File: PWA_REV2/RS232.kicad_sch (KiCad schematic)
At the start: 19 parts

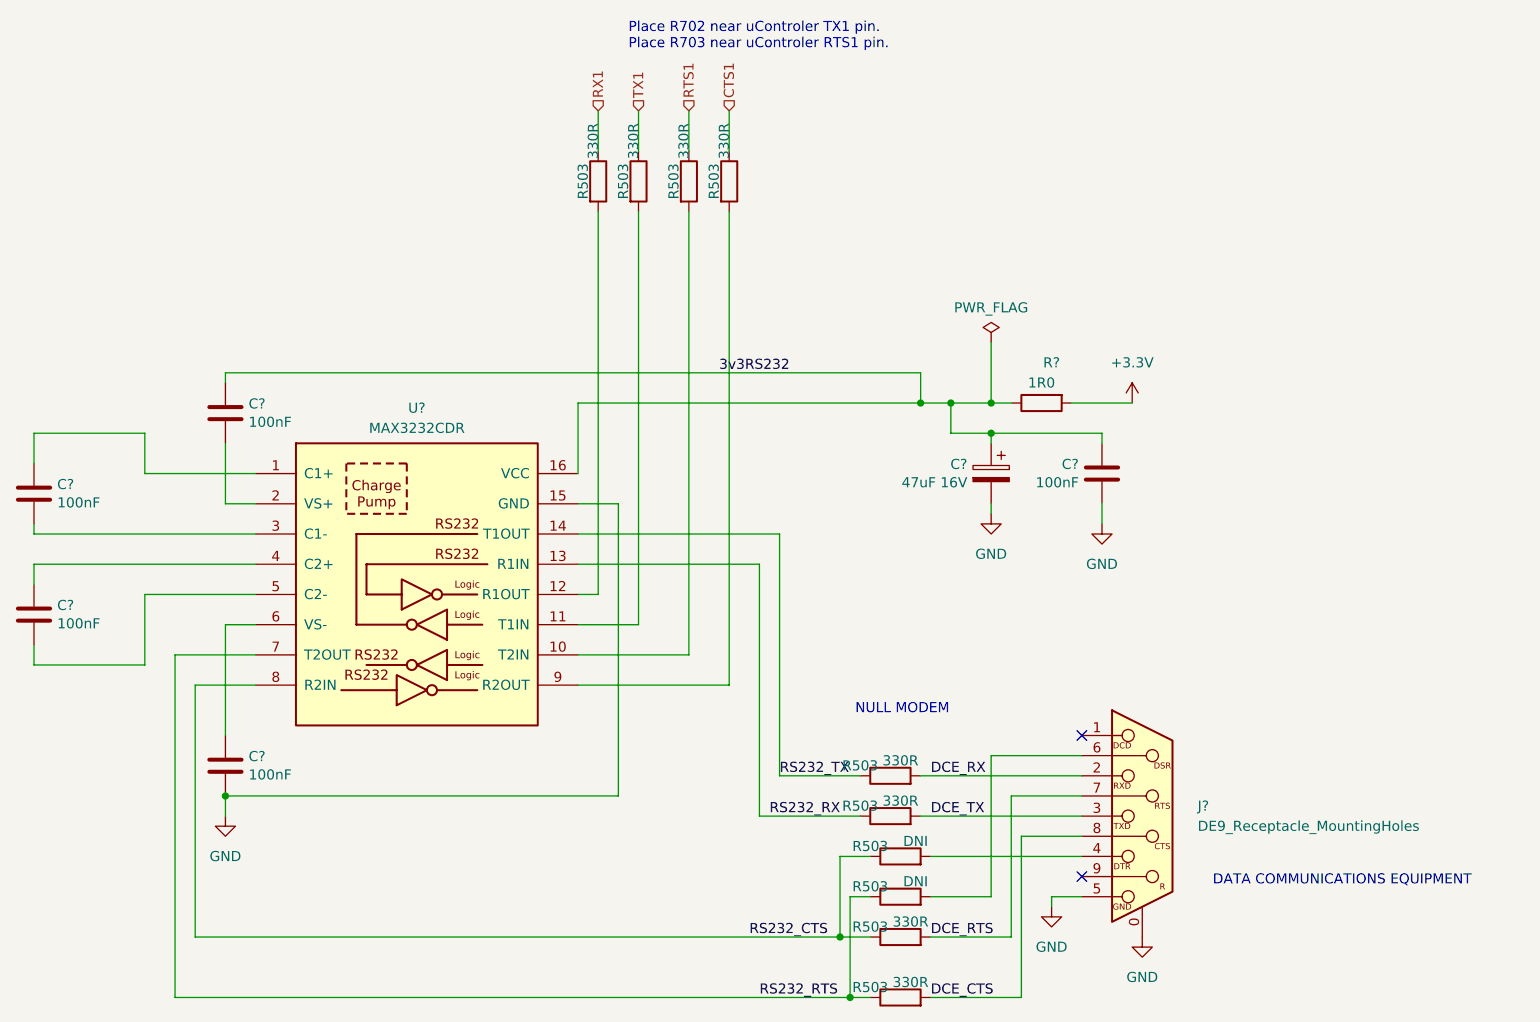
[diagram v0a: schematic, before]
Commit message: Hardware, PWA, Add a Jumper to BOM for J102 so that USB Connector Can Power Krake, issue 312.
:q
q
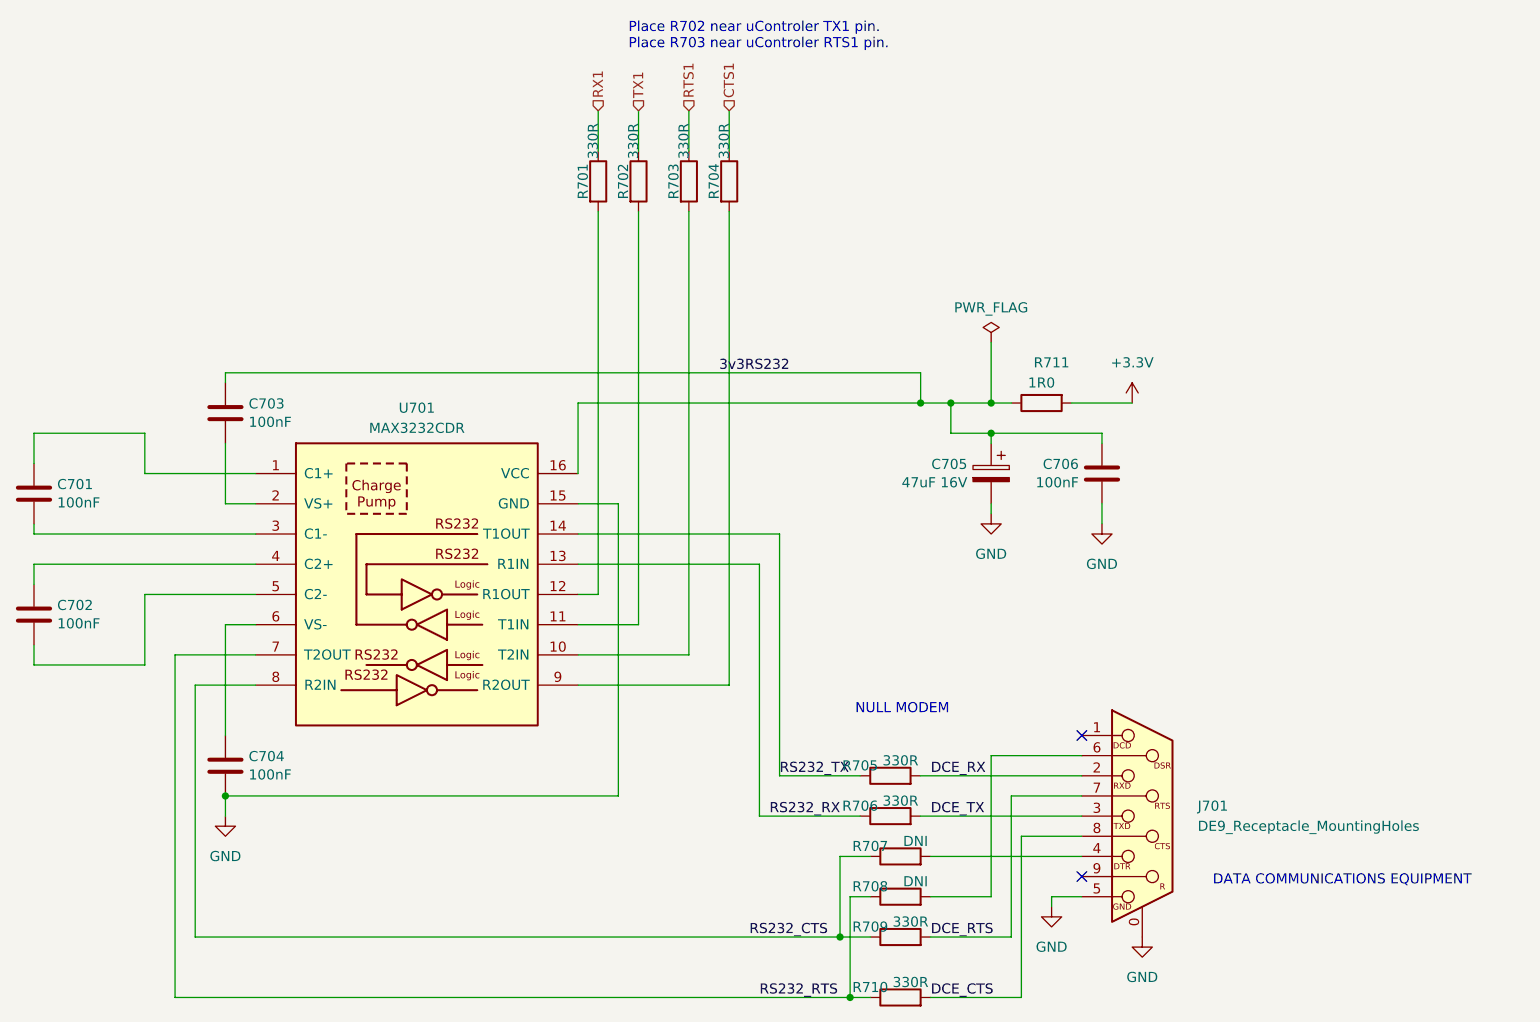
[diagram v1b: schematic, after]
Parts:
- gave numbers to parts that had none: 9
- renumbered R503 to R701, R503 to R702, R503 to R703, R503 to R704, R503 to R705, R503 to R706, R503 to R707, R503 to R708, R503 to R709, R503 to R710

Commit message: Revert "Hardware, PWA, Add a Jumper to BOM for J102 so that USB Connector Can Power Krake, issue 312."
This reverts commit c2819b8ee4999f733f52d823f88f6aefd6456fcc.
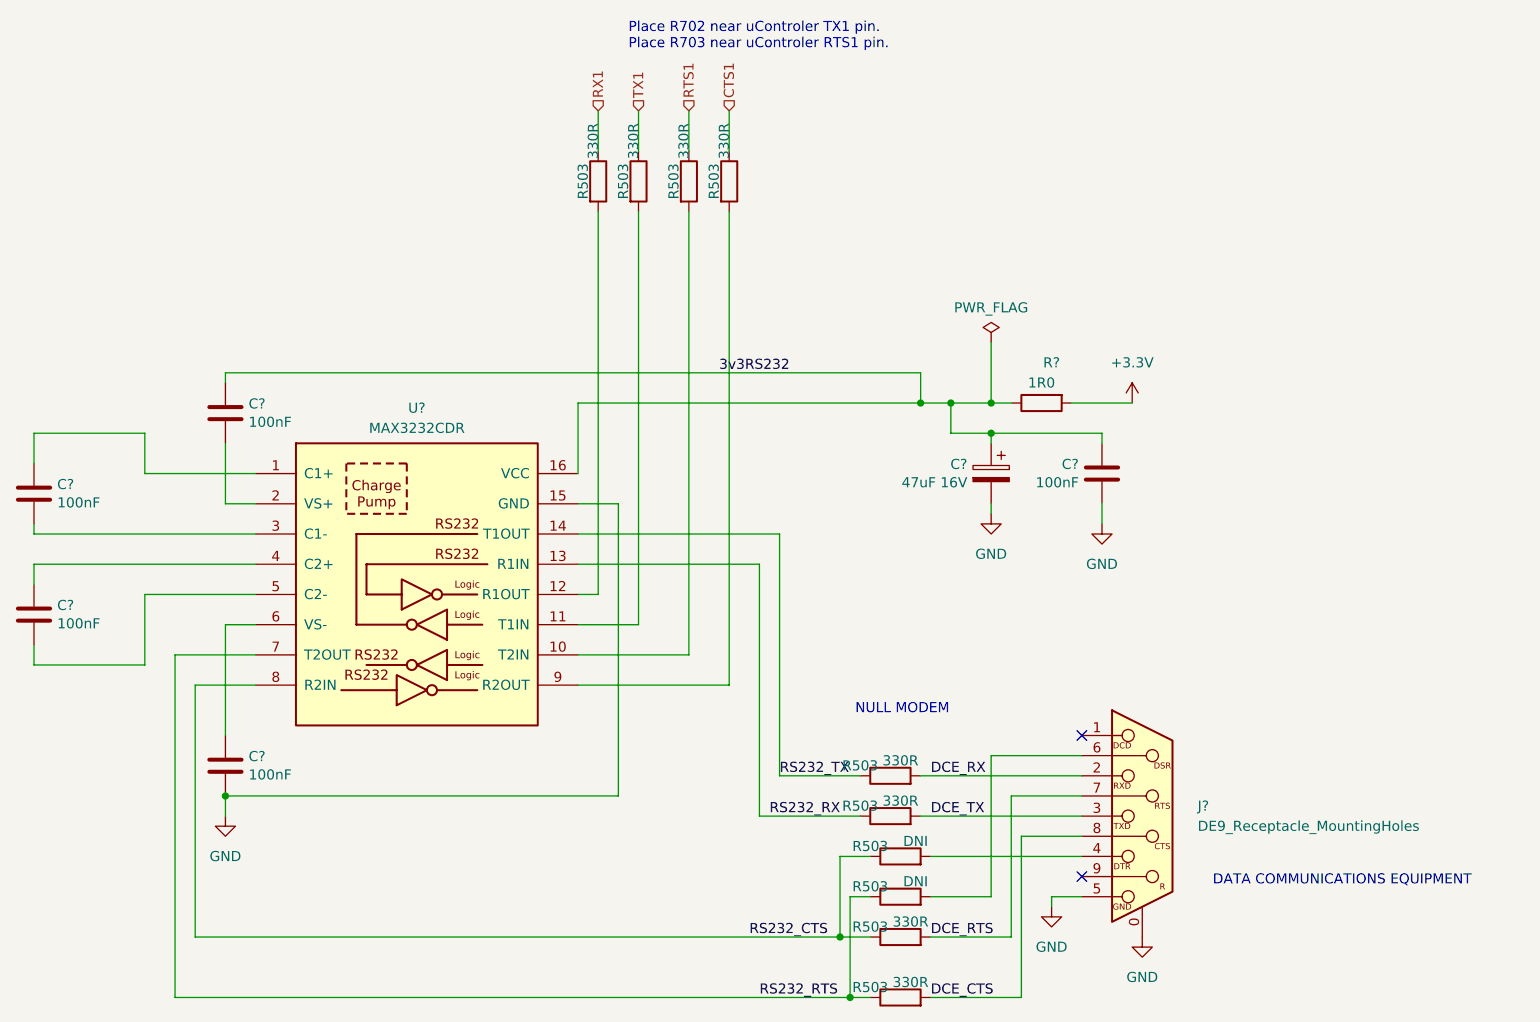
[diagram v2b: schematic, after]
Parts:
- renumbered C705 to C?, C706 to C?, C701 to C?, C702 to C?, C704 to C?, C703 to C?, J701 to J?, R702 to R503, R707 to R503, R710 to R503, R703 to R503, R704 to R503, R706 to R503, R709 to R503, R708 to R503, R701 to R503, R705 to R503, R711 to R?, U701 to U?
